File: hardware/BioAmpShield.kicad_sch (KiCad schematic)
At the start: 50 parts, among them J1 Conn_01x03, J2 SJ1-3525N, J3 Conn_01x03, J4 Conn_01x02, P1 Power, P2 Analog, P3 Digital, P4 Digital, SW1 SW_Push, SW2 SW_Push, U2 TL074

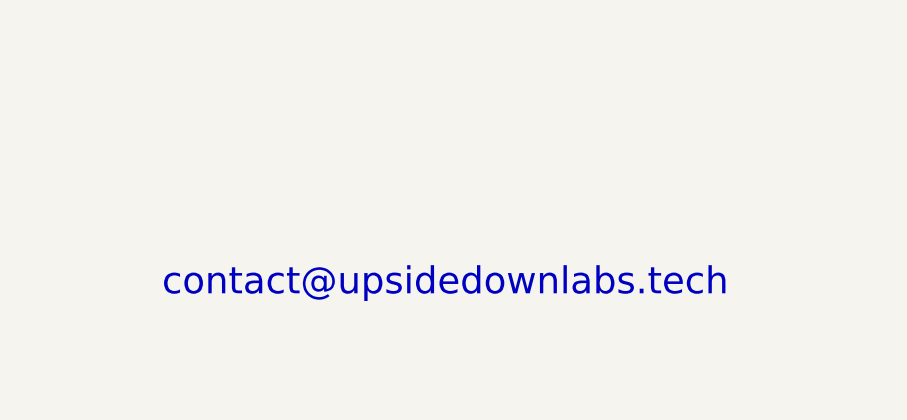
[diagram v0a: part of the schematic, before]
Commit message: Update final design
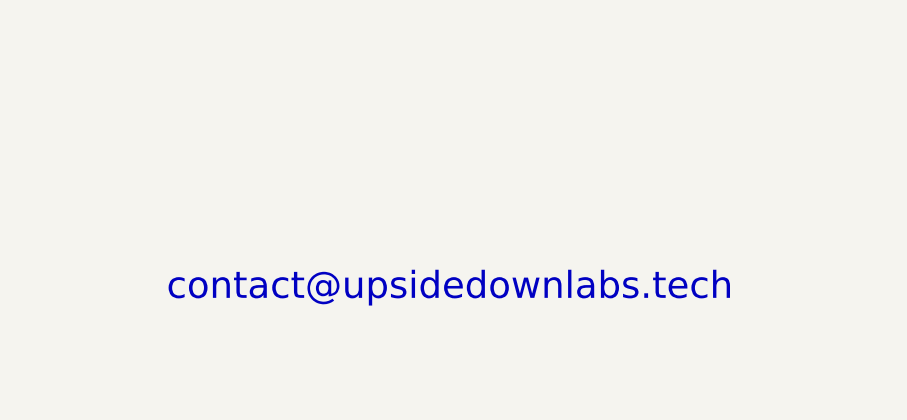
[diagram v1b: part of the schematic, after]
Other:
- company: (none) -> Upside Down Labs
- title: (none) -> Muscle BioAmp Shield
